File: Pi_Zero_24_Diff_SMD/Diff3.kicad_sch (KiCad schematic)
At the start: 14 parts, among them J10 Diff Out, J9 Diff Out, U10 AM26C31, U9 AM26C31

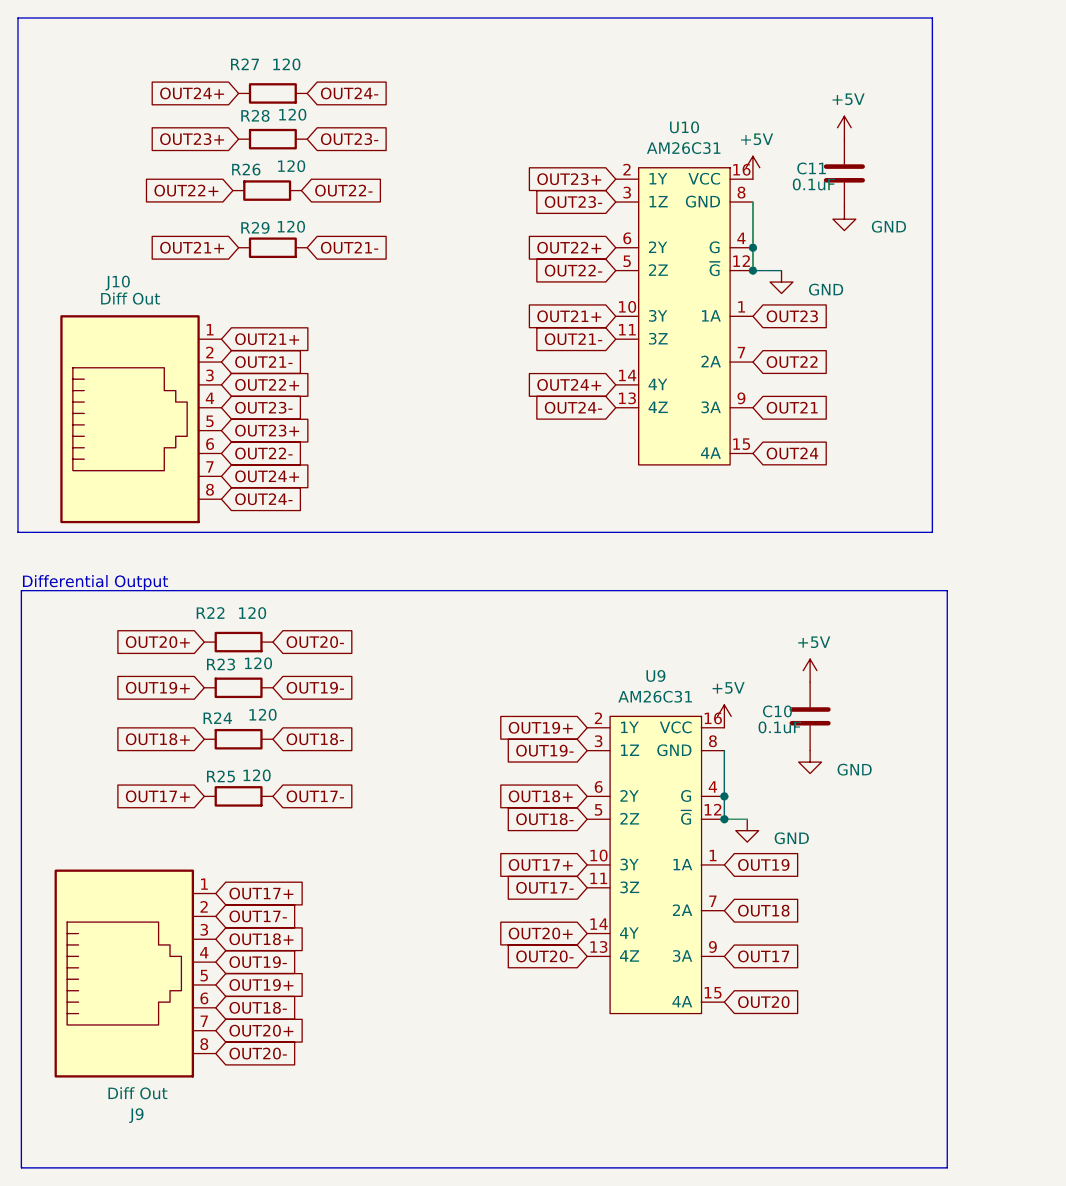
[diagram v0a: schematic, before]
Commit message: working on routing
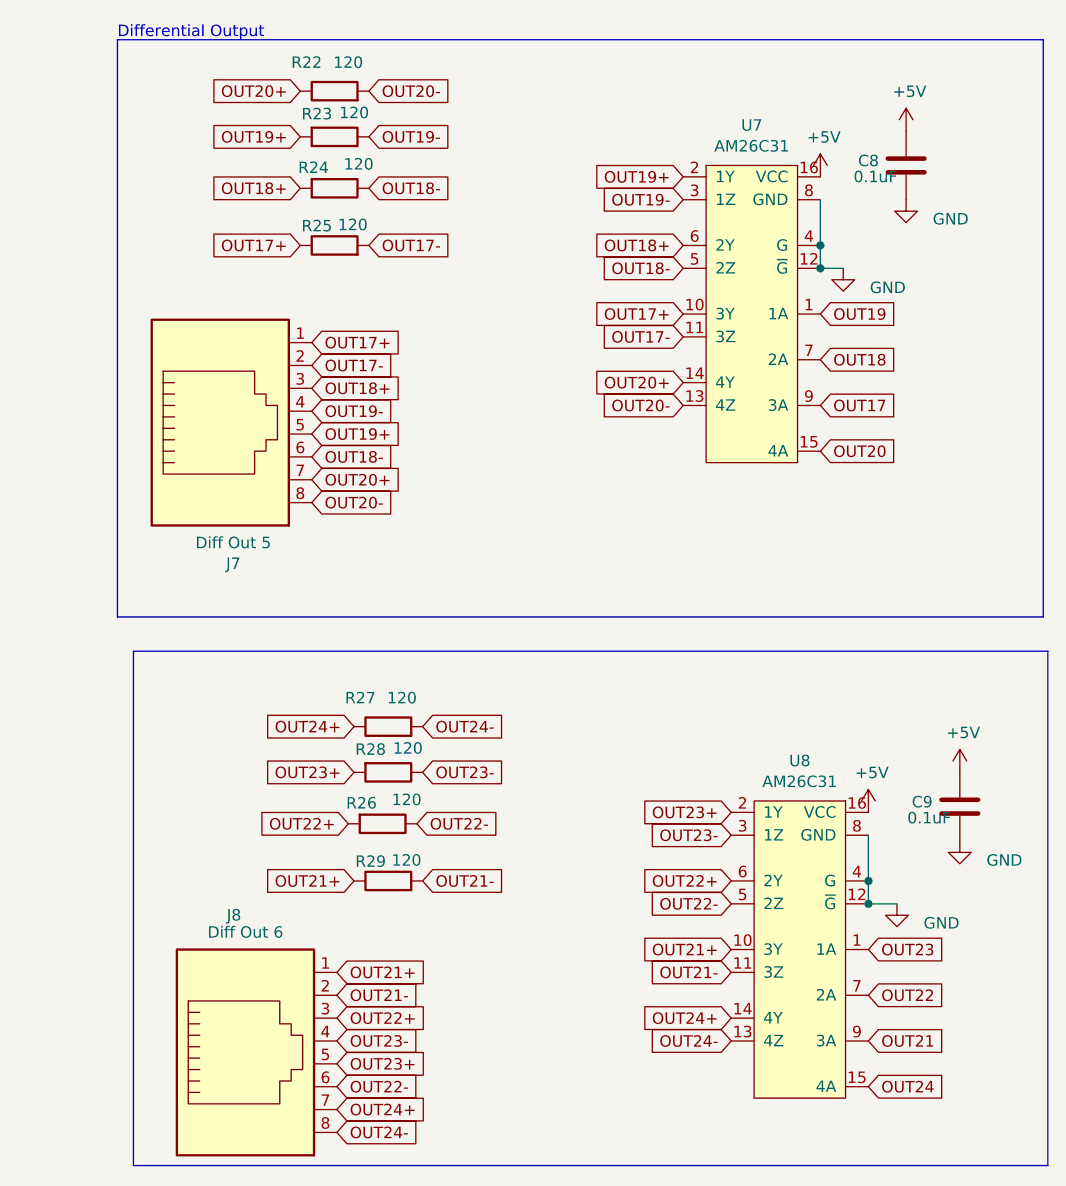
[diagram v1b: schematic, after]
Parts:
- J7: renamed from J9; value Diff Out -> Diff Out 5
- J8: renamed from J10; value Diff Out -> Diff Out 6
- renumbered C10 to C8, C11 to C9, U9 to U7, U10 to U8
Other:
- moved on the sheet: C8, C9, J7, J8, R22, R23, R24, R25, R26, R27, R28, R29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
